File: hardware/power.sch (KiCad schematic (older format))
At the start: 14 parts

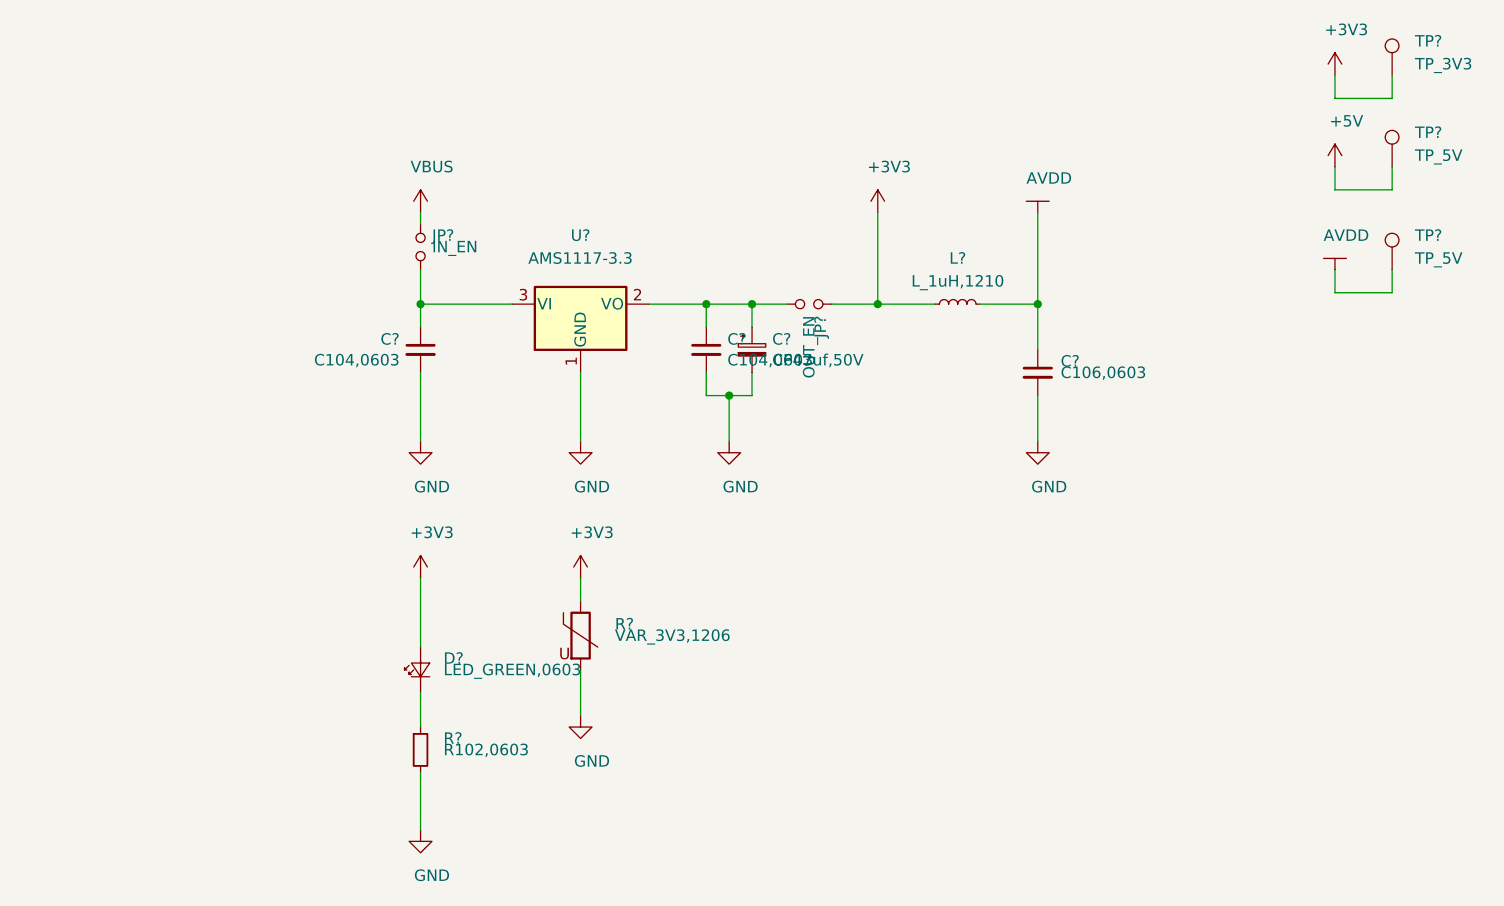
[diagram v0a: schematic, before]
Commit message: update,
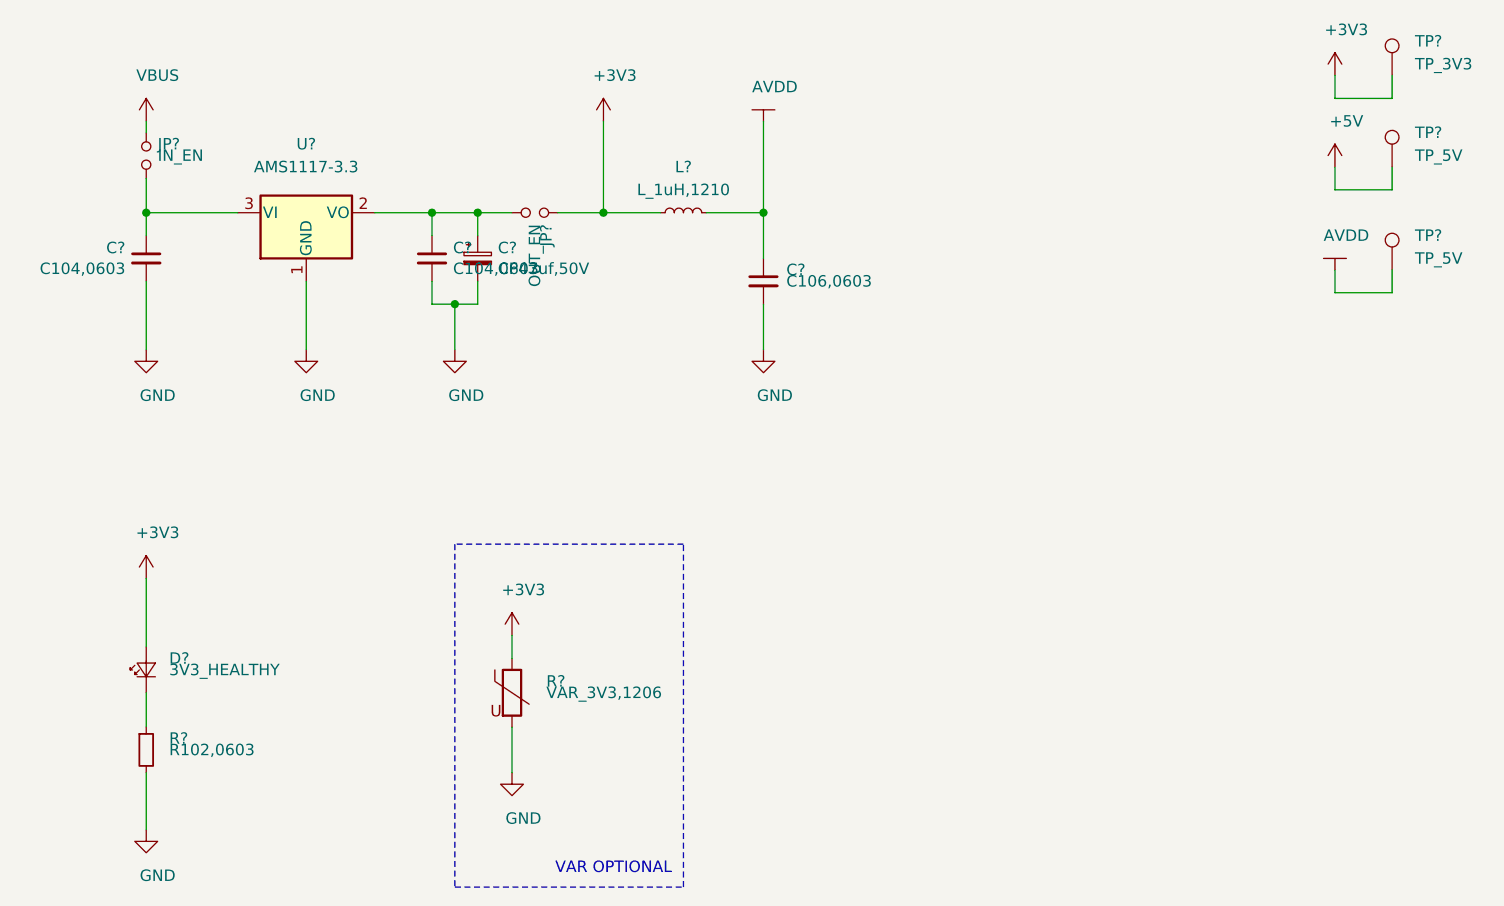
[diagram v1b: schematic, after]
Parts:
- D?: value LED_GREEN,0603 -> 3V3_HEALTHY
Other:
- note added: "VAR OPTIONAL"
- moved on the sheet: C?, D?, JP?, L?, R?, U?
